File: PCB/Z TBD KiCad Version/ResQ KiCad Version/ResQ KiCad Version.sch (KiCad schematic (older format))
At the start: 7 parts

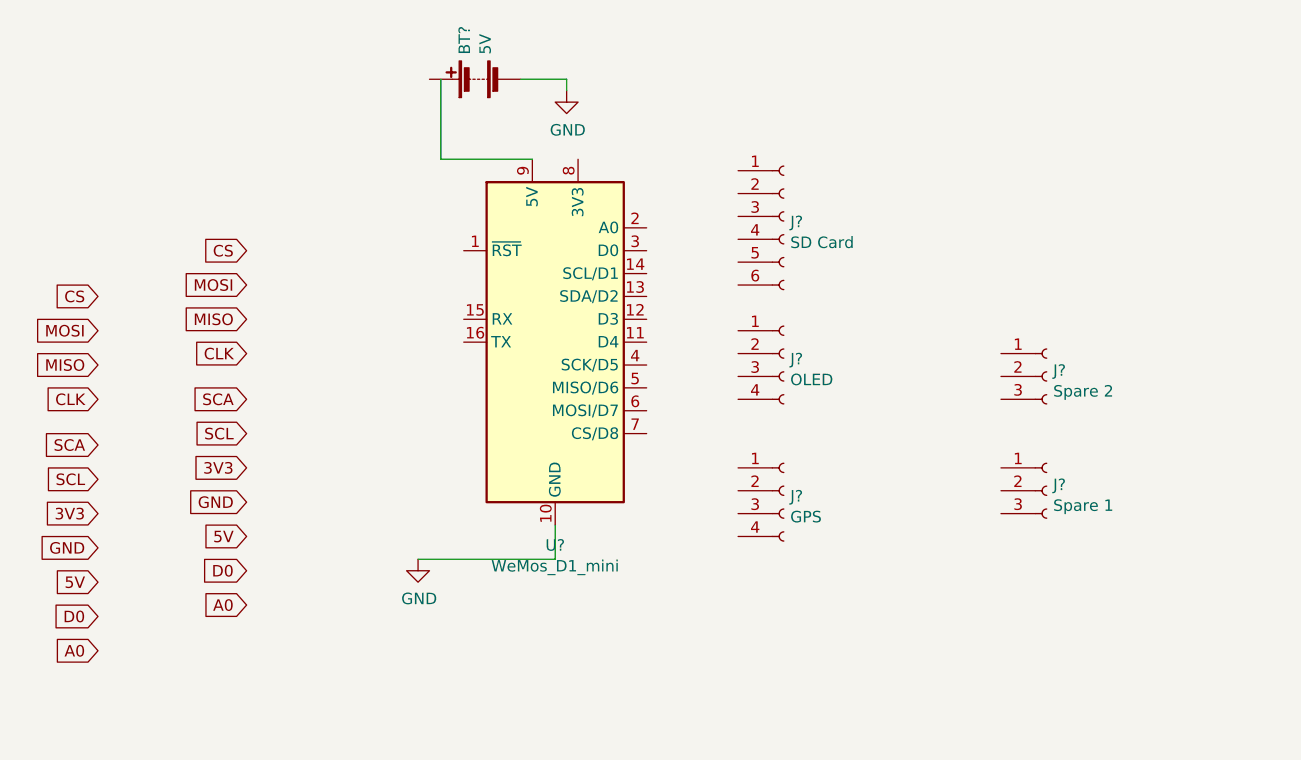
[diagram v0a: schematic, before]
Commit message: KiCad Updates
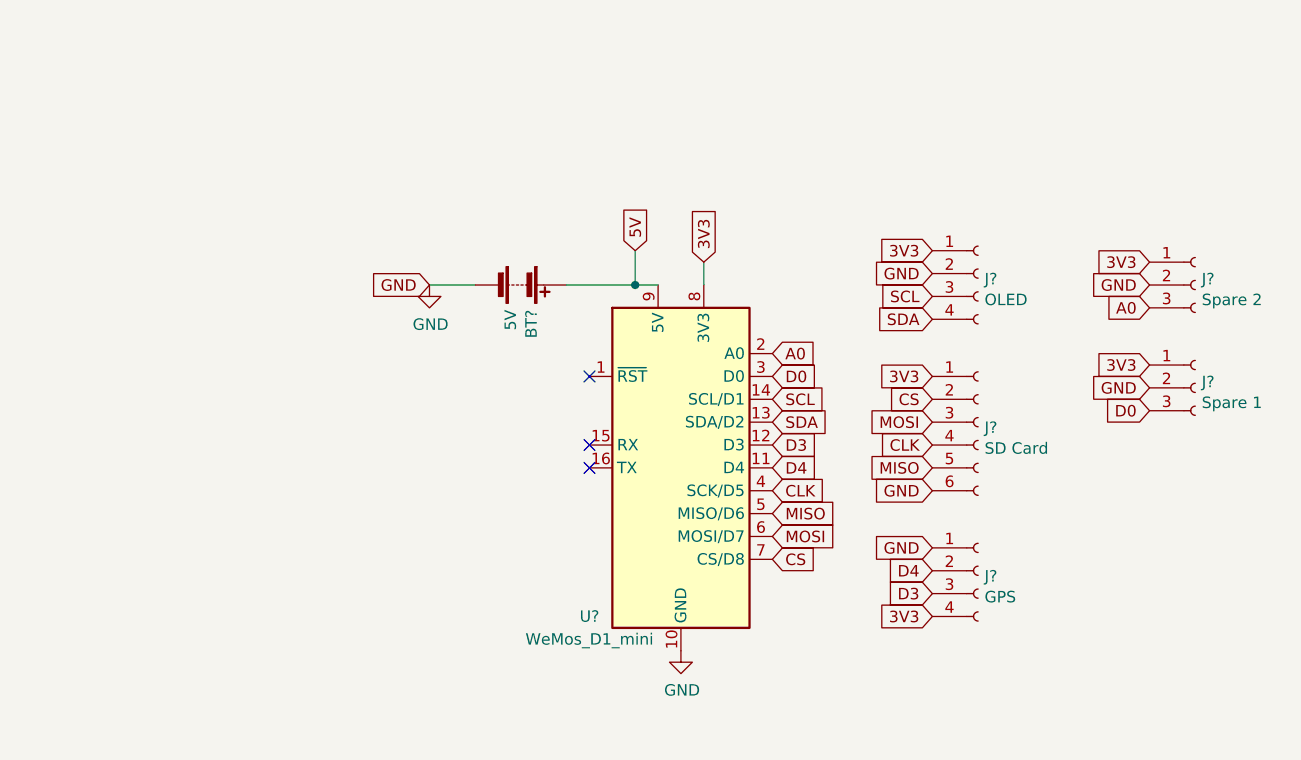
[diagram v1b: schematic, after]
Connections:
- net labels added: D3, D4, SDA
- net labels removed: SCA
- wire segments 6 -> 5
- no-connect marks 0 -> 3
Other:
- moved on the sheet: BT?, J?, U?
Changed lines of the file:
@@
 $EndDescr
-$Comp
-L MCU_Module:WeMos_D1_mini U?
-U 1 1 5F31691B
-P 7250 4750
-F 0 "U?" H 7250 3861 50  0000 C CNN
-F 1 "WeMos_D1_mini" H 7250 3770 50  0000 C CNN
-F 2 "Module:WEMOS_D1_mini_light" H 7250 3600 50  0001 C CNN
-F 3 "https://wiki.wemos.cc/products:d1:d1_mini#documentation" H 5400 3600 50  0001 C CNN
-	1    7250 4750
-	1    0    0    -1
-$EndComp
-$Comp
-L Device:Battery BT?
-U 1 1 5F31A8A9
-P 6900 3600
-F 0 "BT?" H 7008 3646 50  0000 L CNN
-F 1 "5V" H 7008 3555 50  0000 L CNN
-F 2 "" V 6900 3660 50  0001 C CNN
-F 3 "~" V 6900 3660 50  0001 C CNN
-	1    6900 3600
-	0    -1   -1   0
-$EndComp
 $Comp
 L Connector:Conn_01x06_Female J?
 U 1 1 5F31DE3A
-P 8250 4200
-F 0 "J?" H 8278 4176 50  0000 L CNN
-F 1 "SD Card" H 8278 4085 50  0000 L CNN
-F 2 "" H 8250 4200 50  0001 C CNN
-F 3 "~" H 8250 4200 50  0001 C CNN
-	1    8250 4200
+P 9100 5100
+F 0 "J?" H 9128 5076 50  0000 L CNN
+F 1 "SD Card" H 9128 4985 50  0000 L CNN
+F 2 "" H 9100 5100 50  0001 C CNN
+F 3 "~" H 9100 5100 50  0001 C CNN
+	1    9100 5100
+	1    0    0    -1
+$EndComp
+Text GLabel 8900 5000 0    50   Input ~ 0
+CS
+Text GLabel 8900 5100 0    50   Input ~ 0
+MOSI
+Text GLabel 8900 5300 0    50   Input ~ 0
+MISO
+Text GLabel 8900 5200 0    50   Input ~ 0
+CLK
+Text GLabel 8200 5100 2    50   Input ~ 0
+SDA
+Text GLabel 8200 5000 2    50   Input ~ 0
+SCL
+Text GLabel 8900 4900 0    50   Input ~ 0
+3V3
+Text GLabel 8900 5400 0    50   Input ~ 0
+GND
+Text GLabel 8200 4900 2    50   Input ~ 0
+D0
+Text GLabel 8200 4800 2    50   Input ~ 0
+A0
+Text GLabel 8200 5700 2    50   Input ~ 0
+CS
+Text GLabel 8200 5600 2    50   Input ~ 0
+MOSI
+Text GLabel 8200 5500 2    50   Input ~ 0
+MISO
+Text GLabel 8200 5400 2    50   Input ~ 0
+CLK
+Text GLabel 8900 4650 0    50   Input ~ 0
+SDA
+Text GLabel 8900 4550 0    50   Input ~ 0
+SCL
+Text GLabel 7900 4400 1    50   Input ~ 0
+3V3
+Text GLabel 8900 5650 0    50   Input ~ 0
+GND
+Text GLabel 9850 4600 0    50   Input ~ 0
+A0
+Text GLabel 8900 5950 0    50   Input ~ 0
+3V3
+Text GLabel 9850 4850 0    50   Input ~ 0
+3V3
+Text GLabel 8900 4350 0    50   Input ~ 0
+3V3
+Text GLabel 8900 4450 0    50   Input ~ 0
+GND
+Text GLabel 8900 5750 0    50   Input ~ 0
+D4
+Text GLabel 8200 5300 2    50   Input ~ 0
+D4
+Text GLabel 8200 5200 2    50   Input ~ 0
+D3
+Text GLabel 8900 5850 0    50   Input ~ 0
+D3
+Wire Wire Line
+	7600 4500 7600 4350
+Connection ~ 7600 4500
+Wire Wire Line
+	7600 4500 7700 4500
+$Comp
+L power:GND #PWR?
+U 1 1 5F34FDAC
+P 7800 6100
+F 0 "#PWR?" H 7800 5850 50  0001 C CNN
+F 1 "GND" H 7805 5927 50  0000 C CNN
+F 2 "" H 7800 6100 50  0001 C CNN
+F 3 "" H 7800 6100 50  0001 C CNN
+	1    7800 6100
 	1    0    0    -1
 $EndComp
@@
 L Connector:Conn_01x04_Female J?
 U 1 1 5F31F299
-P 8250 4800
-F 0 "J?" H 8278 4776 50  0000 L CNN
-F 1 "OLED" H 8278 4685 50  0000 L CNN
-F 2 "" H 8250 4800 50  0001 C CNN
-F 3 "~" H 8250 4800 50  0001 C CNN
-	1    8250 4800
+P 9100 4450
+F 0 "J?" H 9128 4426 50  0000 L CNN
+F 1 "OLED" H 9128 4335 50  0000 L CNN
+F 2 "" H 9100 4450 50  0001 C CNN
+F 3 "~" H 9100 4450 50  0001 C CNN
+	1    9100 4450
 	1    0    0    -1
 $EndComp
@@
 L Connector:Conn_01x04_Female J?
 U 1 1 5F321884
-P 8250 5400
-F 0 "J?" H 8278 5376 50  0000 L CNN
-F 1 "GPS" H 8278 5285 50  0000 L CNN
-F 2 "" H 8250 5400 50  0001 C CNN
-F 3 "~" H 8250 5400 50  0001 C CNN
-	1    8250 5400
+P 9100 5750
+F 0 "J?" H 9128 5726 50  0000 L CNN
+F 1 "GPS" H 9128 5635 50  0000 L CNN
+F 2 "" H 9100 5750 50  0001 C CNN
+F 3 "~" H 9100 5750 50  0001 C CNN
+	1    9100 5750
+	1    0    0    -1
+$EndComp
+Text GLabel 9850 4500 0    50   Input ~ 0
+GND
+Text GLabel 9850 4400 0    50   Input ~ 0
+3V3
+$Comp
+L Connector:Conn_01x03_Female J?
+U 1 1 5F3230C4
+P 10050 4500
+F 0 "J?" H 10078 4526 50  0000 L CNN
+F 1 "Spare 2" H 10078 4435 50  0000 L CNN
+F 2 "" H 10050 4500 50  0001 C CNN
+F 3 "~" H 10050 4500 50  0001 C CNN
+	1    10050 4500
+	1    0    0    -1
+$EndComp
+NoConn ~ 7400 4900
+NoConn ~ 7400 5200
+NoConn ~ 7400 5300
+Text GLabel 7600 4350 1    50   Input ~ 0
+5V
+Wire Wire Line
+	7900 4400 7900 4500
+Wire Wire Line
+	7300 4500 7600 4500
+$Comp
+L Device:Battery BT?
+U 1 1 5F31A8A9
+P 7100 4500
+F 0 "BT?" H 7208 4546 50  0000 L CNN
+F 1 "5V" H 7208 4455 50  0000 L CNN
+F 2 "" V 7100 4560 50  0001 C CNN
+F 3 "~" V 7100 4560 50  0001 C CNN
+	1    7100 4500
+	0    1    1    0
+$EndComp
+$Comp
+L power:GND #PWR?
+U 1 1 5F34EF30
+P 6700 4500
+F 0 "#PWR?" H 6700 4250 50  0001 C CNN
+F 1 "GND" H 6705 4327 50  0000 C CNN
+F 2 "" H 6700 4500 50  0001 C CNN
+F 3 "" H 6700 4500 50  0001 C CNN
+	1    6700 4500
+	1    0    0    -1
+$EndComp
+Text GLabel 6700 4500 0    50   Input ~ 0
+GND
+Wire Wire Line
+	6900 4500 6700 4500
+Text GLabel 9850 4950 0    50   Input ~ 0
+GND
+Text GLabel 9850 5050 0    50   Input ~ 0
+D0
+$Comp
+L Connector:Conn_01x03_Female J?
+U 1 1 5F322635
+P 10050 4950
+F 0 "J?" H 10078 4976 50  0000 L CNN
+F 1 "Spare 1" H 10078 4885 50  0000 L CNN
+F 2 "" H 10050 4950 50  0001 C CNN
+F 3 "~" H 10050 4950 50  0001 C CNN
+	1    10050 4950
 	1    0    0    -1
 $EndComp
 $Comp
-L Connector:Conn_01x03_Female J?
-U 1 1 5F322635
-P 9400 5400
-F 0 "J?" H 9428 5426 50  0000 L CNN
-F 1 "Spare 1" H 9428 5335 50  0000 L CNN
-F 2 "" H 9400 5400 50  0001 C CNN
-F 3 "~" H 9400 5400 50  0001 C CNN
-	1    9400 5400
+L MCU_Module:WeMos_D1_mini U?
+U 1 1 5F31691B
+P 7800 5300
+F 0 "U?" H 7400 4650 50  0000 C CNN
+F 1 "WeMos_D1_mini" H 7400 4550 50  0000 C CNN
+F 2 "Module:WEMOS_D1_mini_light" H 7800 4150 50  0001 C CNN
+F 3 "https://wiki.wemos.cc/products:d1:d1_mini#documentation" H 5950 4150 50  0001 C CNN
+	1    7800 5300
 	1    0    0    -1
 $EndComp
-$Comp
-L Connector:Conn_01x03_Female J?
-U 1 1 5F3230C4
-P 9400 4900
-F 0 "J?" H 9428 4926 50  0000 L CNN
-F 1 "Spare 2" H 9428 4835 50  0000 L CNN
-F 2 "" H 9400 4900 50  0001 C CNN
-F 3 "~" H 9400 4900 50  0001 C CNN
-	1    9400 4900
-	1    0    0    -1
-$EndComp
-Wire Wire Line
-	6750 3600 6750 3950
-Wire Wire Line
-	6750 3950 7150 3950
-$Comp
-L power:GND #PWR?
-U 1 1 5F34EF30
-P 7300 3650
-F 0 "#PWR?" H 7300 3400 50  0001 C CNN
-F 1 "GND" H 7305 3477 50  0000 C CNN
-F 2 "" H 7300 3650 50  0001 C CNN
-F 3 "" H 7300 3650 50  0001 C CNN
-	1    7300 3650
-	1    0    0    -1
-$EndComp
-Wire Wire Line
-	7100 3600 7300 3600
-Wire Wire Line
-	7300 3600 7300 3650
-$Comp
-L power:GND #PWR?
-U 1 1 5F34FDAC
-P 6650 5700
-F 0 "#PWR?" H 6650 5450 50  0001 C CNN
-F 1 "GND" H 6655 5527 50  0000 C CNN
-F 2 "" H 6650 5700 50  0001 C CNN
-F 3 "" H 6650 5700 50  0001 C CNN
-	1    6650 5700
-	1    0    0    -1
-$EndComp
-Wire Wire Line
-	6650 5700 7250 5700
-Wire Wire Line
-	7250 5700 7250 5550
-Text GLabel 5250 4550 0    50   Input ~ 0
-CS
-Text GLabel 5250 4700 0    50   Input ~ 0
-MOSI
-Text GLabel 5250 4850 0    50   Input ~ 0
-MISO
-Text GLabel 5250 5000 0    50   Input ~ 0
-CLK
-Text GLabel 5250 5200 0    50   Input ~ 0
-SCA
-Text GLabel 5250 5350 0    50   Input ~ 0
-SCL
-Text GLabel 5250 5500 0    50   Input ~ 0
-3V3
-Text GLabel 5250 5650 0    50   Input ~ 0
-GND
-Text GLabel 5250 5800 0    50   Input ~ 0
-5V
-Text GLabel 5250 5950 0    50   Input ~ 0
-D0
-Text GLabel 5250 6100 0    50   Input ~ 0
-A0
-Text GLabel 5900 4350 0    50   Input ~ 0
-CS
-Text GLabel 5900 4500 0    50   Input ~ 0
-MOSI
-Text GLabel 5900 4650 0    50   Input ~ 0
-MISO
-Text GLabel 5900 4800 0    50   Input ~ 0
-CLK
-Text GLabel 5900 5000 0    50   Input ~ 0
-SCA
-Text GLabel 5900 5150 0    50   Input ~ 0
-SCL
-Text GLabel 5900 5300 0    50   Input ~ 0
-3V3
-Text GLabel 5900 5450 0    50   Input ~ 0
-GND
-Text GLabel 5900 5600 0    50   Input ~ 0
-5V
-Text GLabel 5900 5750 0    50   Input ~ 0
-D0
-Text GLabel 5900 5900 0    50   Input ~ 0
-A0
 $EndSCHEMATC

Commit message: up
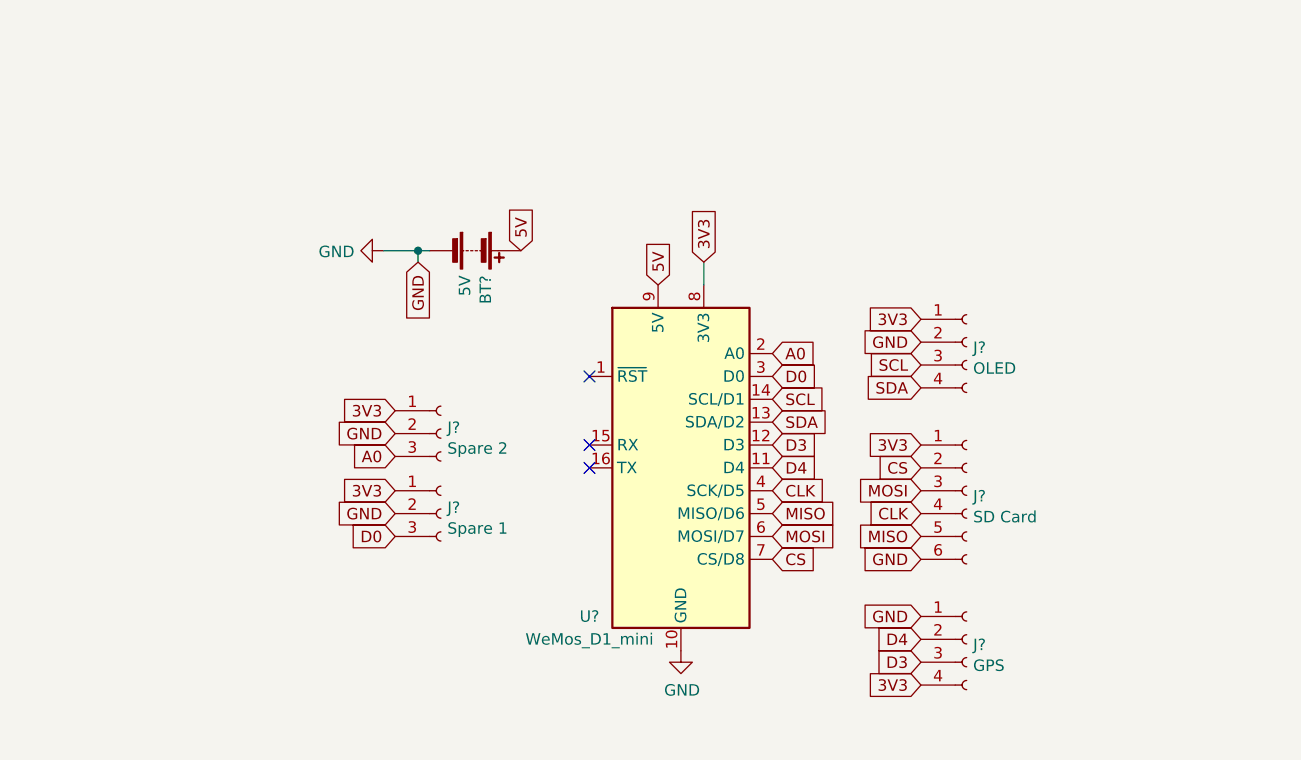
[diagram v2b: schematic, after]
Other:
- moved on the sheet: BT?, J?
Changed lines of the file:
@@
 L Connector:Conn_01x06_Female J?
 U 1 1 5F31DE3A
-P 9100 5100
-F 0 "J?" H 9128 5076 50  0000 L CNN
-F 1 "SD Card" H 9128 4985 50  0000 L CNN
-F 2 "" H 9100 5100 50  0001 C CNN
-F 3 "~" H 9100 5100 50  0001 C CNN
-	1    9100 5100
+P 9050 5400
+F 0 "J?" H 9078 5376 50  0000 L CNN
+F 1 "SD Card" H 9078 5285 50  0000 L CNN
+F 2 "" H 9050 5400 50  0001 C CNN
+F 3 "~" H 9050 5400 50  0001 C CNN
+	1    9050 5400
 	1    0    0    -1
 $EndComp
-Text GLabel 8900 5000 0    50   Input ~ 0
+Text GLabel 8850 5300 0    50   Input ~ 0
 CS
-Text GLabel 8900 5100 0    50   Input ~ 0
+Text GLabel 8850 5400 0    50   Input ~ 0
 MOSI
-Text GLabel 8900 5300 0    50   Input ~ 0
+Text GLabel 8850 5600 0    50   Input ~ 0
 MISO
-Text GLabel 8900 5200 0    50   Input ~ 0
+Text GLabel 8850 5500 0    50   Input ~ 0
 CLK
 Text GLabel 8200 5100 2    50   Input ~ 0
@@
 Text GLabel 8200 5000 2    50   Input ~ 0
 SCL
-Text GLabel 8900 4900 0    50   Input ~ 0
+Text GLabel 8850 5200 0    50   Input ~ 0
 3V3
-Text GLabel 8900 5400 0    50   Input ~ 0
+Text GLabel 8850 5700 0    50   Input ~ 0
 GND
 Text GLabel 8200 4900 2    50   Input ~ 0
@@
 Text GLabel 8200 5400 2    50   Input ~ 0
 CLK
-Text GLabel 8900 4650 0    50   Input ~ 0
+Text GLabel 8850 4950 0    50   Input ~ 0
 SDA
-Text GLabel 8900 4550 0    50   Input ~ 0
+Text GLabel 8850 4850 0    50   Input ~ 0
 SCL
 Text GLabel 7900 4400 1    50   Input ~ 0
 3V3
-Text GLabel 8900 5650 0    50   Input ~ 0
+Text GLabel 8850 5950 0    50   Input ~ 0
 GND
-Text GLabel 9850 4600 0    50   Input ~ 0
-A0
-Text GLabel 8900 5950 0    50   Input ~ 0
+Text GLabel 8850 6250 0    50   Input ~ 0
 3V3
-Text GLabel 9850 4850 0    50   Input ~ 0
+Text GLabel 8850 4650 0    50   Input ~ 0
 3V3
-Text GLabel 8900 4350 0    50   Input ~ 0
-3V3
-Text GLabel 8900 4450 0    50   Input ~ 0
+Text GLabel 8850 4750 0    50   Input ~ 0
 GND
-Text GLabel 8900 5750 0    50   Input ~ 0
+Text GLabel 8850 6050 0    50   Input ~ 0
 D4
 Text GLabel 8200 5300 2    50   Input ~ 0
@@
 Text GLabel 8200 5200 2    50   Input ~ 0
 D3
-Text GLabel 8900 5850 0    50   Input ~ 0
+Text GLabel 8850 6150 0    50   Input ~ 0
 D3
-Wire Wire Line
-	7600 4500 7600 4350
-Connection ~ 7600 4500
-Wire Wire Line
-	7600 4500 7700 4500
 $Comp
 L power:GND #PWR?
@@
 L Connector:Conn_01x04_Female J?
 U 1 1 5F31F299
-P 9100 4450
-F 0 "J?" H 9128 4426 50  0000 L CNN
-F 1 "OLED" H 9128 4335 50  0000 L CNN
-F 2 "" H 9100 4450 50  0001 C CNN
-F 3 "~" H 9100 4450 50  0001 C CNN
-	1    9100 4450
+P 9050 4750
+F 0 "J?" H 9078 4726 50  0000 L CNN
+F 1 "OLED" H 9078 4635 50  0000 L CNN
+F 2 "" H 9050 4750 50  0001 C CNN
+F 3 "~" H 9050 4750 50  0001 C CNN
+	1    9050 4750
 	1    0    0    -1
 $EndComp
@@
 L Connector:Conn_01x04_Female J?
 U 1 1 5F321884
-P 9100 5750
-F 0 "J?" H 9128 5726 50  0000 L CNN
-F 1 "GPS" H 9128 5635 50  0000 L CNN
-F 2 "" H 9100 5750 50  0001 C CNN
-F 3 "~" H 9100 5750 50  0001 C CNN
-	1    9100 5750
-	1    0    0    -1
-$EndComp
-Text GLabel 9850 4500 0    50   Input ~ 0
-GND
-Text GLabel 9850 4400 0    50   Input ~ 0
-3V3
-$Comp
-L Connector:Conn_01x03_Female J?
-U 1 1 5F3230C4
-P 10050 4500
-F 0 "J?" H 10078 4526 50  0000 L CNN
-F 1 "Spare 2" H 10078 4435 50  0000 L CNN
-F 2 "" H 10050 4500 50  0001 C CNN
-F 3 "~" H 10050 4500 50  0001 C CNN
-	1    10050 4500
+P 9050 6050
+F 0 "J?" H 9078 6026 50  0000 L CNN
+F 1 "GPS" H 9078 5935 50  0000 L CNN
+F 2 "" H 9050 6050 50  0001 C CNN
+F 3 "~" H 9050 6050 50  0001 C CNN
+	1    9050 6050
 	1    0    0    -1
 $EndComp
@@
 NoConn ~ 7400 5200
 NoConn ~ 7400 5300
-Text GLabel 7600 4350 1    50   Input ~ 0
-5V
 Wire Wire Line
 	7900 4400 7900 4500
+$Comp
+L Connector:Conn_01x03_Female J?
+U 1 1 5F322635
+P 6750 5500
+F 0 "J?" H 6778 5526 50  0000 L CNN
+F 1 "Spare 1" H 6778 5435 50  0000 L CNN
+F 2 "" H 6750 5500 50  0001 C CNN
+F 3 "~" H 6750 5500 50  0001 C CNN
+	1    6750 5500
+	1    0    0    -1
+$EndComp
+Text GLabel 6550 5600 0    50   Input ~ 0
+D0
+Text GLabel 6550 5500 0    50   Input ~ 0
+GND
+$Comp
+L Connector:Conn_01x03_Female J?
+U 1 1 5F3230C4
+P 6750 5150
+F 0 "J?" H 6778 5176 50  0000 L CNN
+F 1 "Spare 2" H 6778 5085 50  0000 L CNN
+F 2 "" H 6750 5150 50  0001 C CNN
+F 3 "~" H 6750 5150 50  0001 C CNN
+	1    6750 5150
+	1    0    0    -1
+$EndComp
+Text GLabel 6550 5050 0    50   Input ~ 0
+3V3
+Text GLabel 6550 5150 0    50   Input ~ 0
+GND
+Text GLabel 6550 5400 0    50   Input ~ 0
+3V3
+Text GLabel 6550 5250 0    50   Input ~ 0
+A0
 Wire Wire Line
-	7300 4500 7600 4500
+	6700 4350 6650 4350
+Text GLabel 6650 4400 3    50   Input ~ 0
+GND
+$Comp
+L power:GND #PWR?
+U 1 1 5F34EF30
+P 6500 4350
+F 0 "#PWR?" H 6500 4100 50  0001 C CNN
+F 1 "GND" V 6505 4222 50  0000 R CNN
+F 2 "" H 6500 4350 50  0001 C CNN
+F 3 "" H 6500 4350 50  0001 C CNN
+	1    6500 4350
+	0    1    1    0
+$EndComp
 $Comp
 L Device:Battery BT?
 U 1 1 5F31A8A9
-P 7100 4500
-F 0 "BT?" H 7208 4546 50  0000 L CNN
-F 1 "5V" H 7208 4455 50  0000 L CNN
-F 2 "" V 7100 4560 50  0001 C CNN
-F 3 "~" V 7100 4560 50  0001 C CNN
-	1    7100 4500
+P 6900 4350
+F 0 "BT?" H 7008 4396 50  0000 L CNN
+F 1 "5V" H 7008 4305 50  0000 L CNN
+F 2 "" V 6900 4410 50  0001 C CNN
+F 3 "~" V 6900 4410 50  0001 C CNN
+	1    6900 4350
 	0    1    1    0
 $EndComp
-$Comp
-L power:GND #PWR?
-U 1 1 5F34EF30
-P 6700 4500
-F 0 "#PWR?" H 6700 4250 50  0001 C CNN
-F 1 "GND" H 6705 4327 50  0000 C CNN
-F 2 "" H 6700 4500 50  0001 C CNN
-F 3 "" H 6700 4500 50  0001 C CNN
-	1    6700 4500
-	1    0    0    -1
-$EndComp
-Text GLabel 6700 4500 0    50   Input ~ 0
-GND
-Wire Wire Line
-	6900 4500 6700 4500
-Text GLabel 9850 4950 0    50   Input ~ 0
-GND
-Text GLabel 9850 5050 0    50   Input ~ 0
-D0
-$Comp
-L Connector:Conn_01x03_Female J?
-U 1 1 5F322635
-P 10050 4950
-F 0 "J?" H 10078 4976 50  0000 L CNN
-F 1 "Spare 1" H 10078 4885 50  0000 L CNN
-F 2 "" H 10050 4950 50  0001 C CNN
-F 3 "~" H 10050 4950 50  0001 C CNN
-	1    10050 4950
-	1    0    0    -1
-$EndComp
+Text GLabel 7700 4500 1    50   Input ~ 0
+5V
 $Comp
 L MCU_Module:WeMos_D1_mini U?
@@
 	1    0    0    -1
 $EndComp
+Text GLabel 7100 4350 1    50   Input ~ 0
+5V
+Wire Wire Line
+	6650 4350 6650 4400
+Connection ~ 6650 4350
+Wire Wire Line
+	6650 4350 6500 4350
 $EndSCHEMATC
